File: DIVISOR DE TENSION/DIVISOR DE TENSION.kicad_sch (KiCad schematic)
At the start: 12 parts, among them J1 Screw_Terminal_01x02, J2 Conn_01x01_Pin

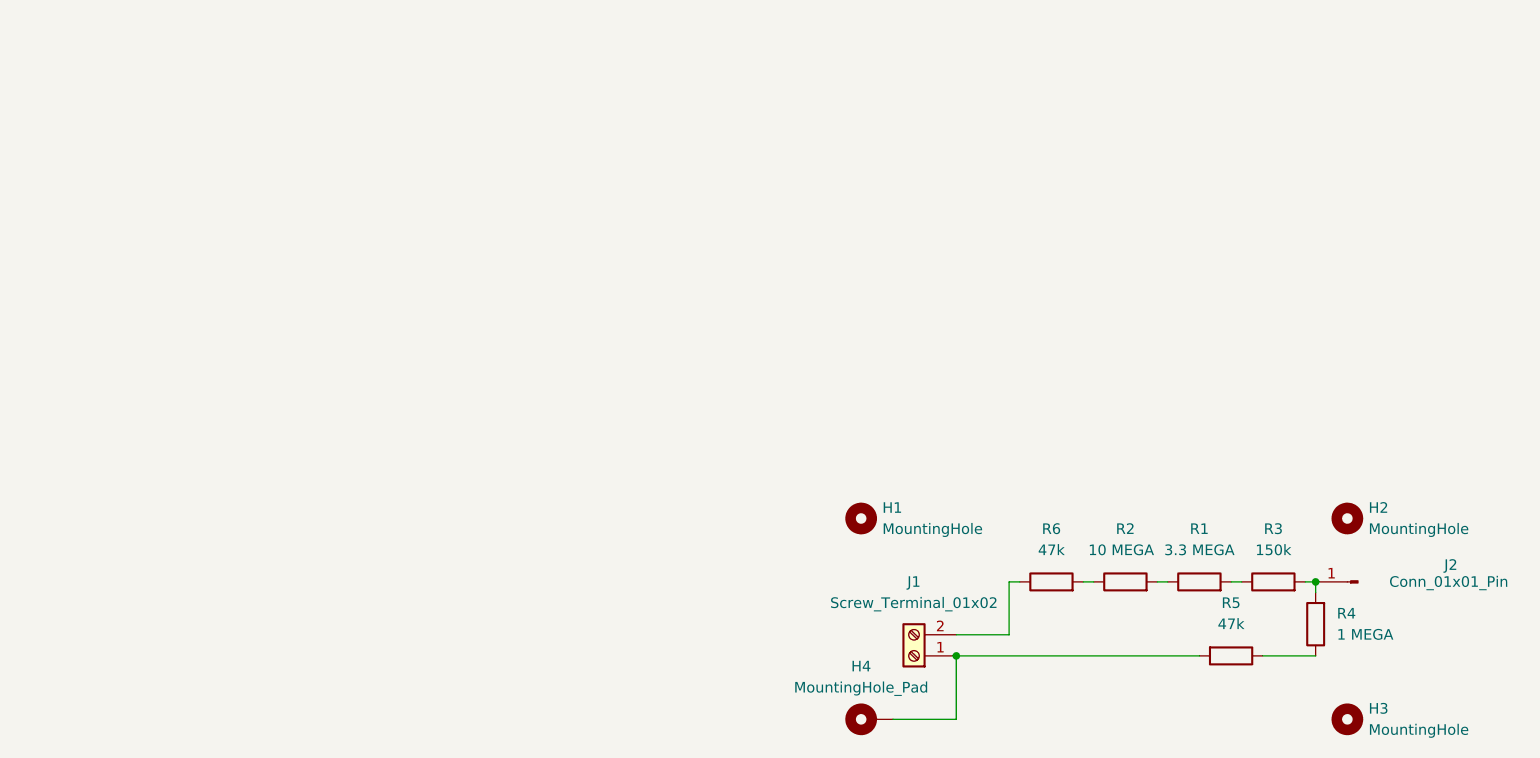
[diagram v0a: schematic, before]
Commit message: FINAL VERSION 2025
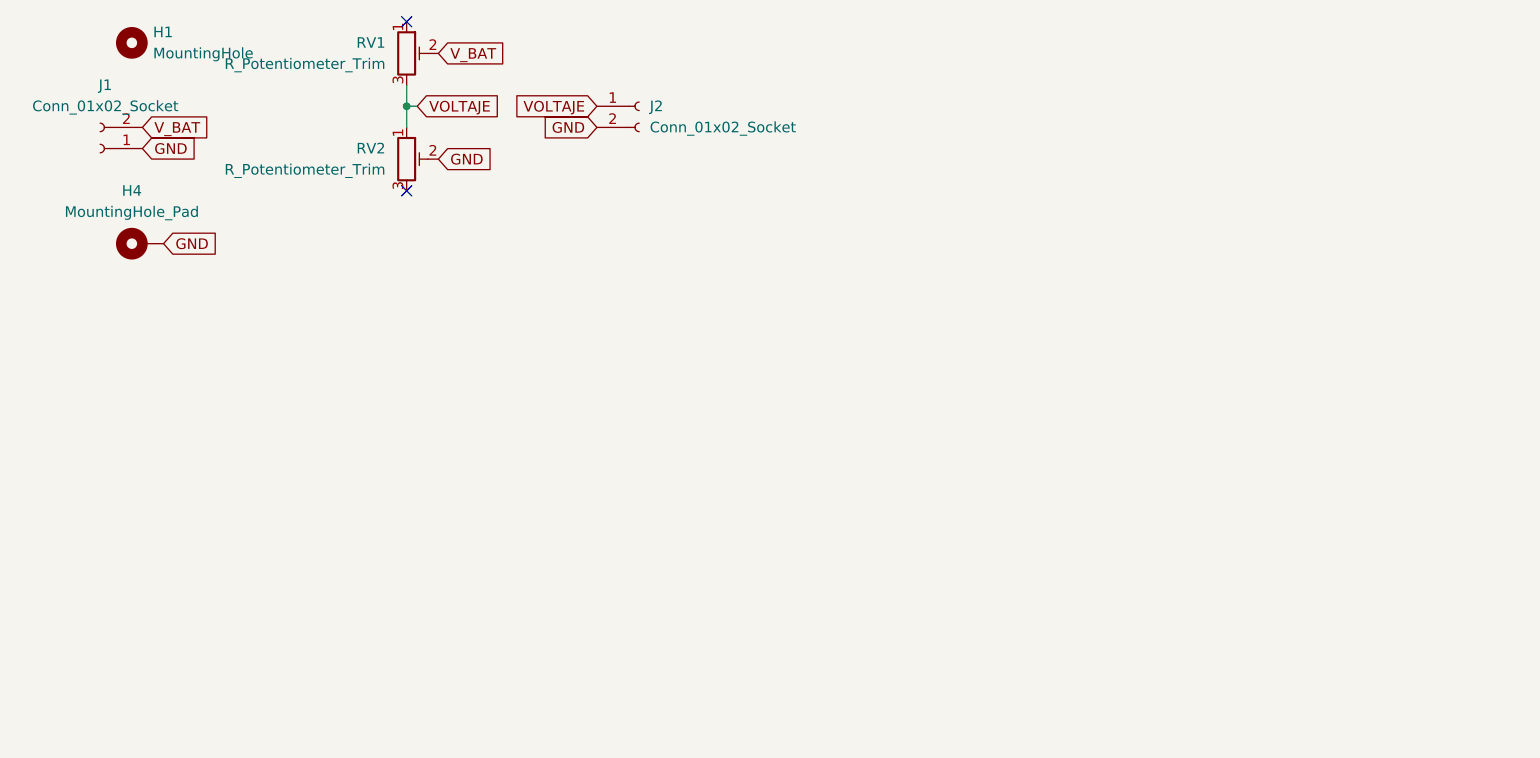
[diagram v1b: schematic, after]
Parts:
- removed H2, H3: MountingHole, MountingHole:MountingHole_2.2mm_M2, symbol Mechanical:MountingHole
- removed J1: Screw_Terminal_01x02, TerminalBlock:TerminalBlock_MaiXu_MX126-5.0-02P_1x02_P5.00mm, symbol Connector:Screw_Terminal_01x02
- removed J2: Conn_01x01_Pin, Connector_Pin:Pin_D0.7mm_L6.5mm_W1.8mm_FlatFork, symbol Connector:Conn_01x01_Pin
- removed R1: 3.3 MEGA, Resistor_THT:R_Axial_DIN0204_L3.6mm_D1.6mm_P7.62mm_Horizontal, symbol Device:R
- removed R2: 10 MEGA, Resistor_THT:R_Axial_DIN0204_L3.6mm_D1.6mm_P7.62mm_Horizontal, symbol Device:R
- removed R3: 150k, Resistor_THT:R_Axial_DIN0204_L3.6mm_D1.6mm_P7.62mm_Horizontal, symbol Device:R
- removed R4: 1 MEGA, Resistor_THT:R_Axial_DIN0204_L3.6mm_D1.6mm_P7.62mm_Horizontal, symbol Device:R
- removed R5, R6: 47k, Resistor_THT:R_Axial_DIN0204_L3.6mm_D1.6mm_P7.62mm_Horizontal, symbol Device:R
- added J1, J2: Conn_01x02_Socket, Connector_JST:JST_EH_B2B-EH-A_1x02_P2.50mm_Vertical, symbol Connector:Conn_01x02_Socket
- added RV1, RV2: R_Potentiometer_Trim, Potentiometer_THT:Potentiometer_Bourns_3266Y_Vertical, symbol Device:R_Potentiometer_Trim
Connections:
- net GND: now reaches H4.1
- net GND: now also J1.1 (Pin_1), J2.2 (Pin_2), RV2.2
- new net VOLTAJE: J2.1 (Pin_1), RV1.3, RV2.1
- new net V_BAT: J1.2 (Pin_2), RV1.2
- no-connect marks 0 -> 2
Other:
- moved on the sheet: H1, H4
